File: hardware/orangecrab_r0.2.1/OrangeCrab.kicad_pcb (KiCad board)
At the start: 6 copper layers, 50.8 x 22.9 mm, 163 parts, among them J1 Conn_01x12_Male, J2 Conn_01x16_Male, J3 USB_C_Receptacle_USB2.0, J4 MicroSd, J5 JST, J6 Conn_01x05_Male, SW1 SW_Push, U1 TLV62569DRL, U10 NCP115-2.5, U2 TLV62569DRL, U3 LFE5U-25F-8MG285C, U4 MT41K64M16TW-107_J-TR, U5 BQ24232, U6 W25Q128JVP, U7 TLV62569DRL, U9 74HC4067BQ

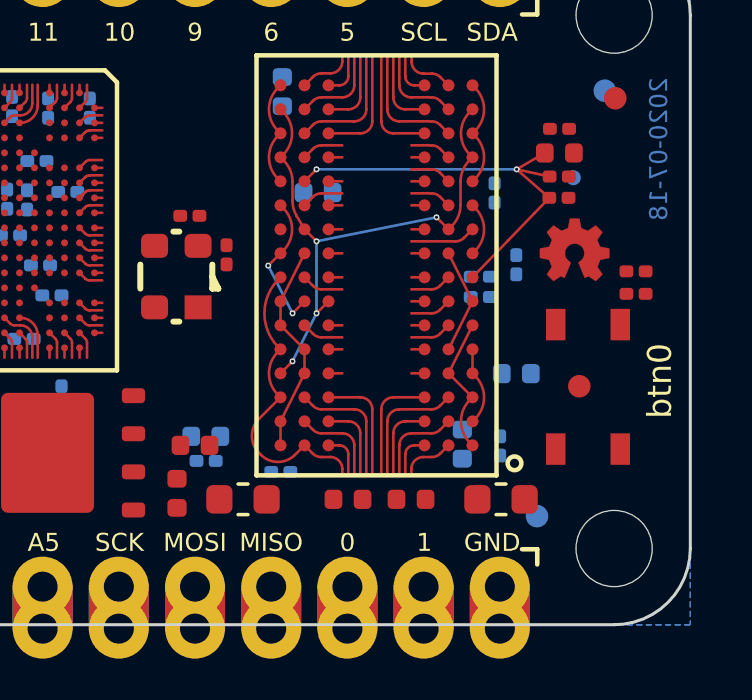
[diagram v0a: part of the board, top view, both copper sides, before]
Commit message: refresh
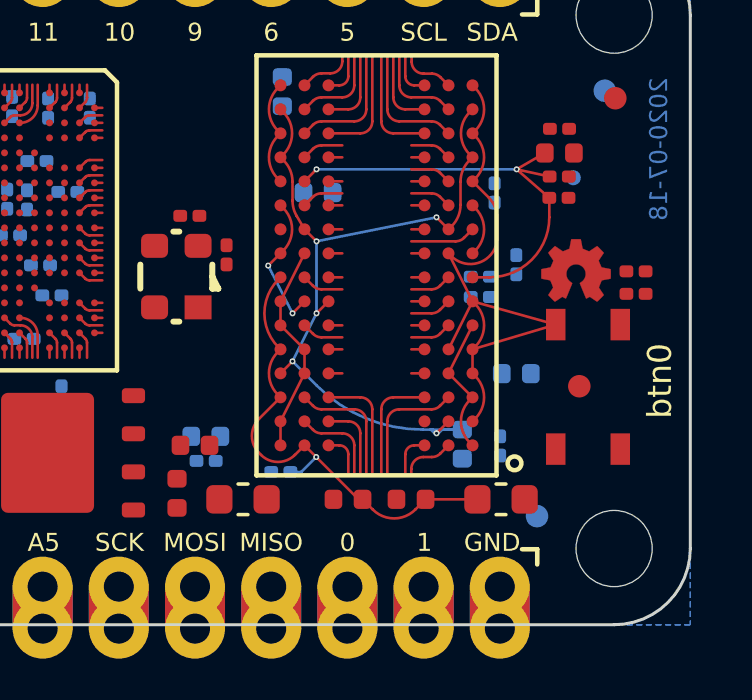
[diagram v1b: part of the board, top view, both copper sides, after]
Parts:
- moved G*** 0.69 mm to (181.5, 102.6)
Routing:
- net GND: track 80.1 -> 89.3 mm
- net /DRAM/RAM_VDDQ: track 16.6 -> 22.8 mm, vias 0 -> 1
- net /DRAM/RAM_VDD: track 22.3 -> 27.9 mm, vias 4 -> 5
- net ECP5_VREF: track 15.4 -> 16.0 mm
